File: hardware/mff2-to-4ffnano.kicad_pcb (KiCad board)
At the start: 2 copper layers, 48 x 13 mm, 2 parts, among them U1 SIM-NANO-4FF, U2 ESIMSON8

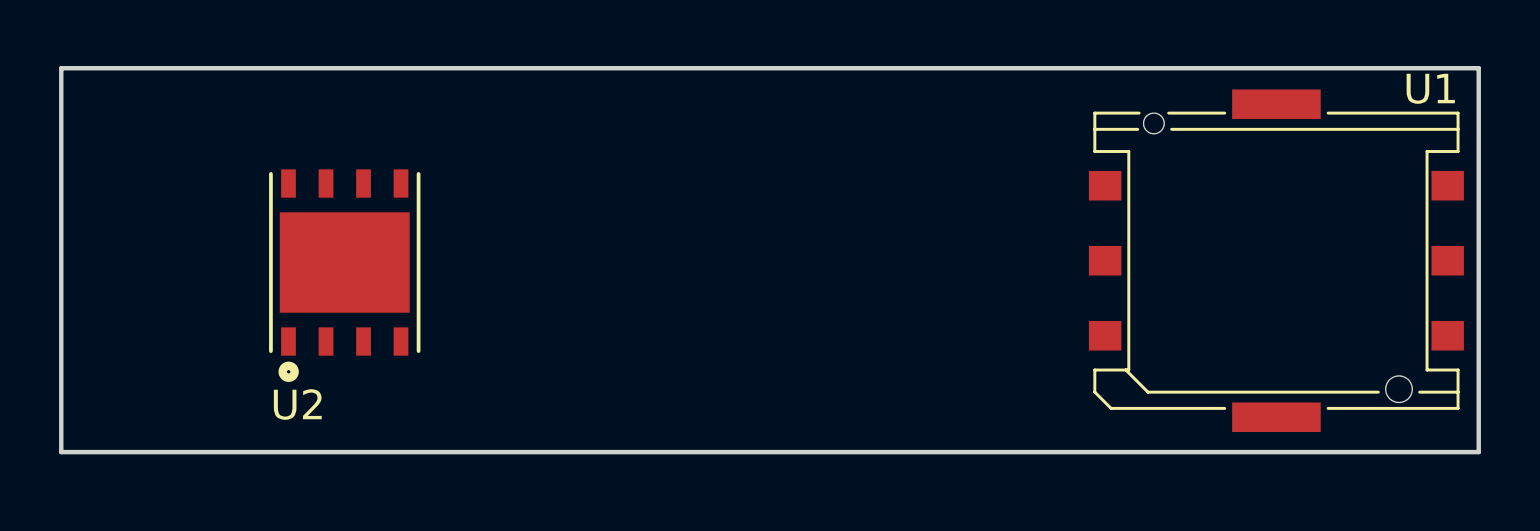
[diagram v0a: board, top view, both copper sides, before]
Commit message: castellated flex design v1.0
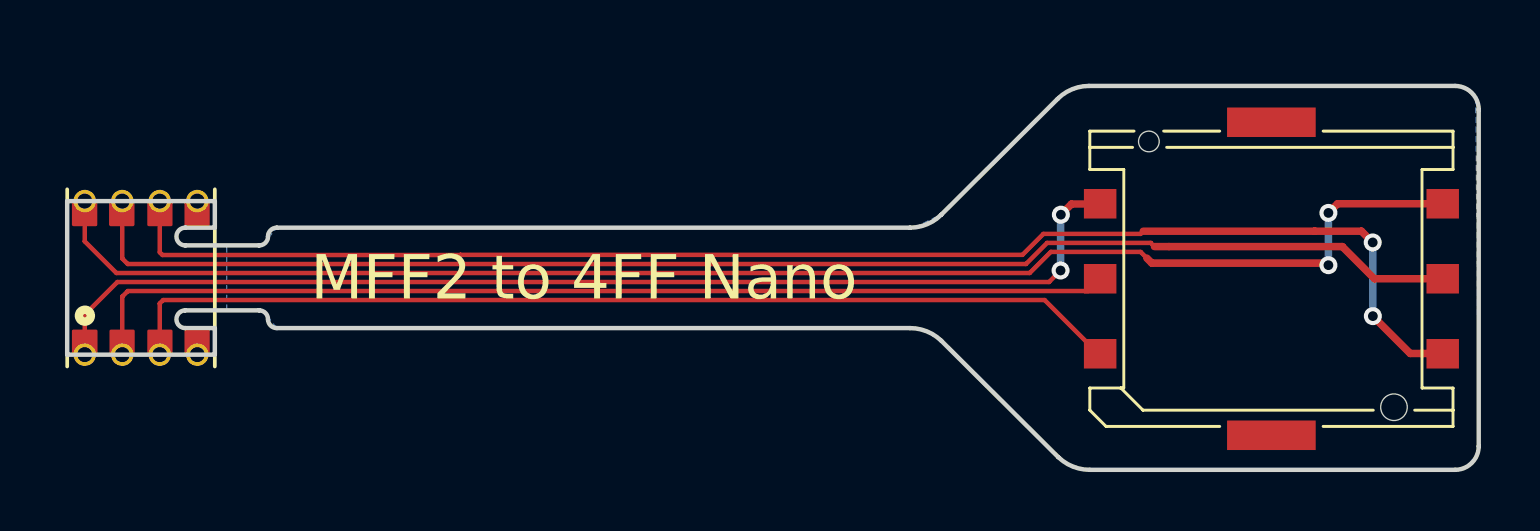
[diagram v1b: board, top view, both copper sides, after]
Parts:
- U2: footprint mff2-to-4ffnano:MFF2 -> mff2-to-4ffnano:MFF2-castellated
- moved U2 6.92 mm to (120.4, 130.9)
- moved U1 0.63 mm to (158.7, 130.9)
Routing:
- net +5V: track 0.00 -> 50.2 mm, vias 0 -> 2
- net CLK: track 0.00 -> 48.5 mm, vias 0 -> 2
- net RST: track 0.00 -> 47.5 mm
- net GND: track 0.00 -> 38.4 mm, vias 0 -> 2
- net VPP: track 0.00 -> 35.3 mm
- net MISO: track 0.00 -> 34.4 mm
- added copper zone on B.Cu, net GND
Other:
- board size 48 x 13 mm -> 47.8 x 13 mm
- net class Default: clearance 0.254 -> 0.1524
- rule trace_clearance: 0.254 -> 0.1524
- board text added: "MFF2 to 4FF Nano"
- board text removed: "TODO: convert this footprint to castellated through-hole"
